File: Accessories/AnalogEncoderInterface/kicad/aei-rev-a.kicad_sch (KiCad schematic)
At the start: 55 parts, among them J1 Screw_Terminal_01x06, J2 1935161, J3 Screw_Terminal_01x06, U1 INA2143U, U2 INA2143U, U3 LT1764EQ-1.5-PBF, U4 RJHSE5380

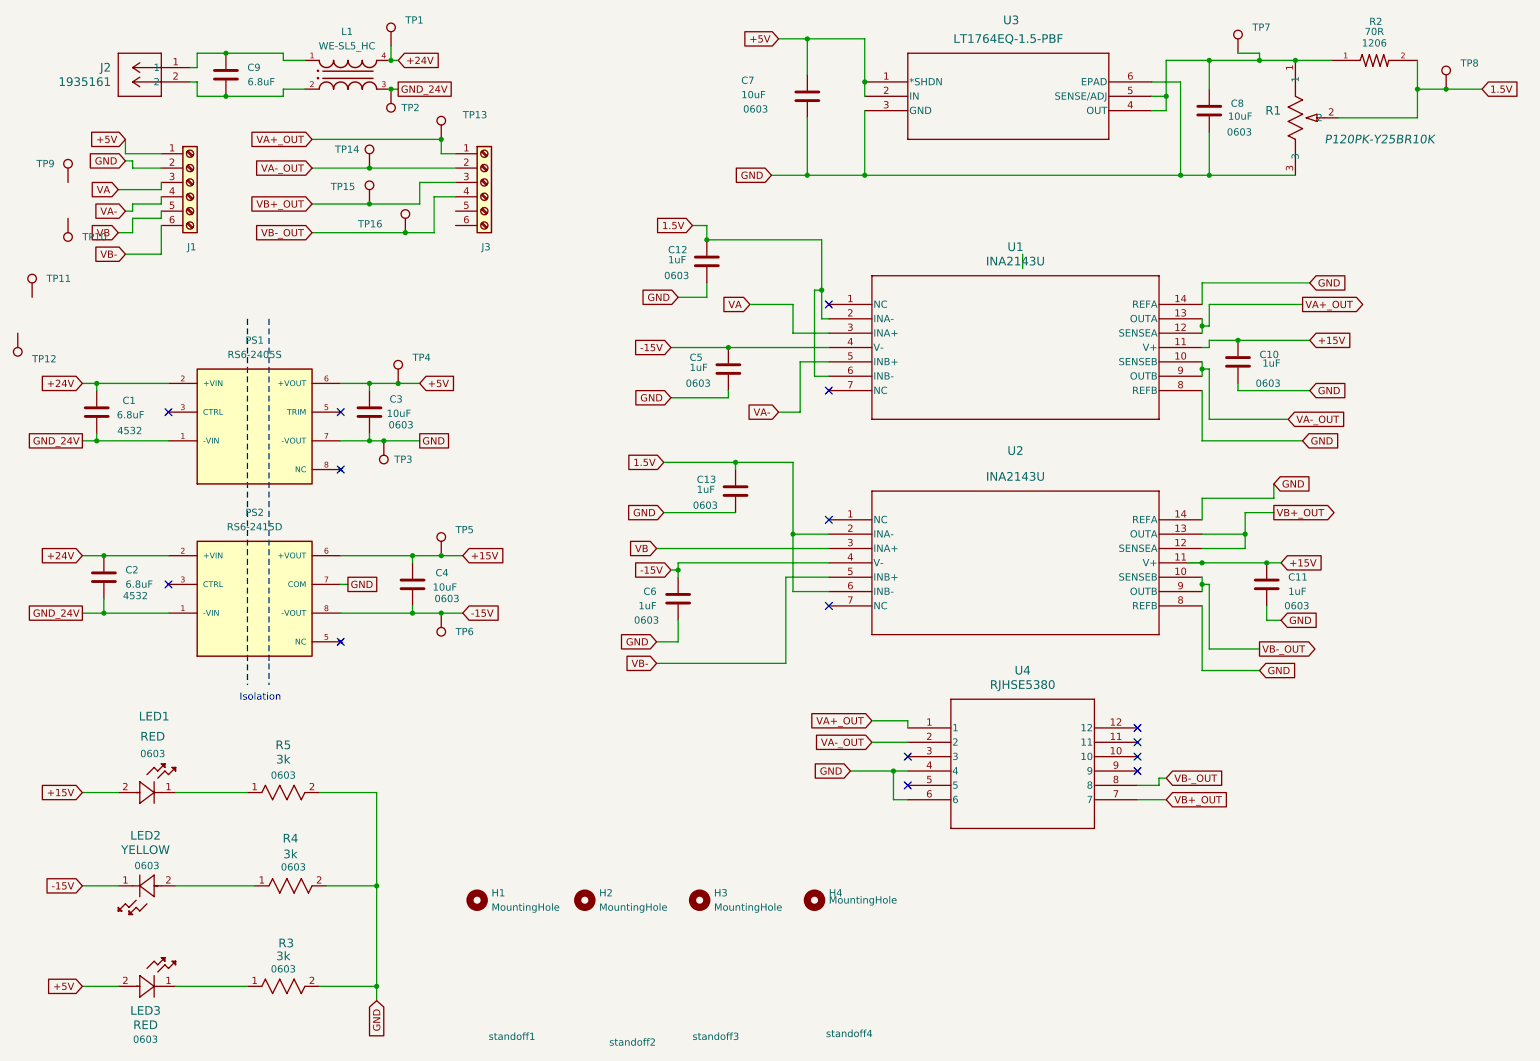
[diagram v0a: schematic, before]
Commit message: update the schematics
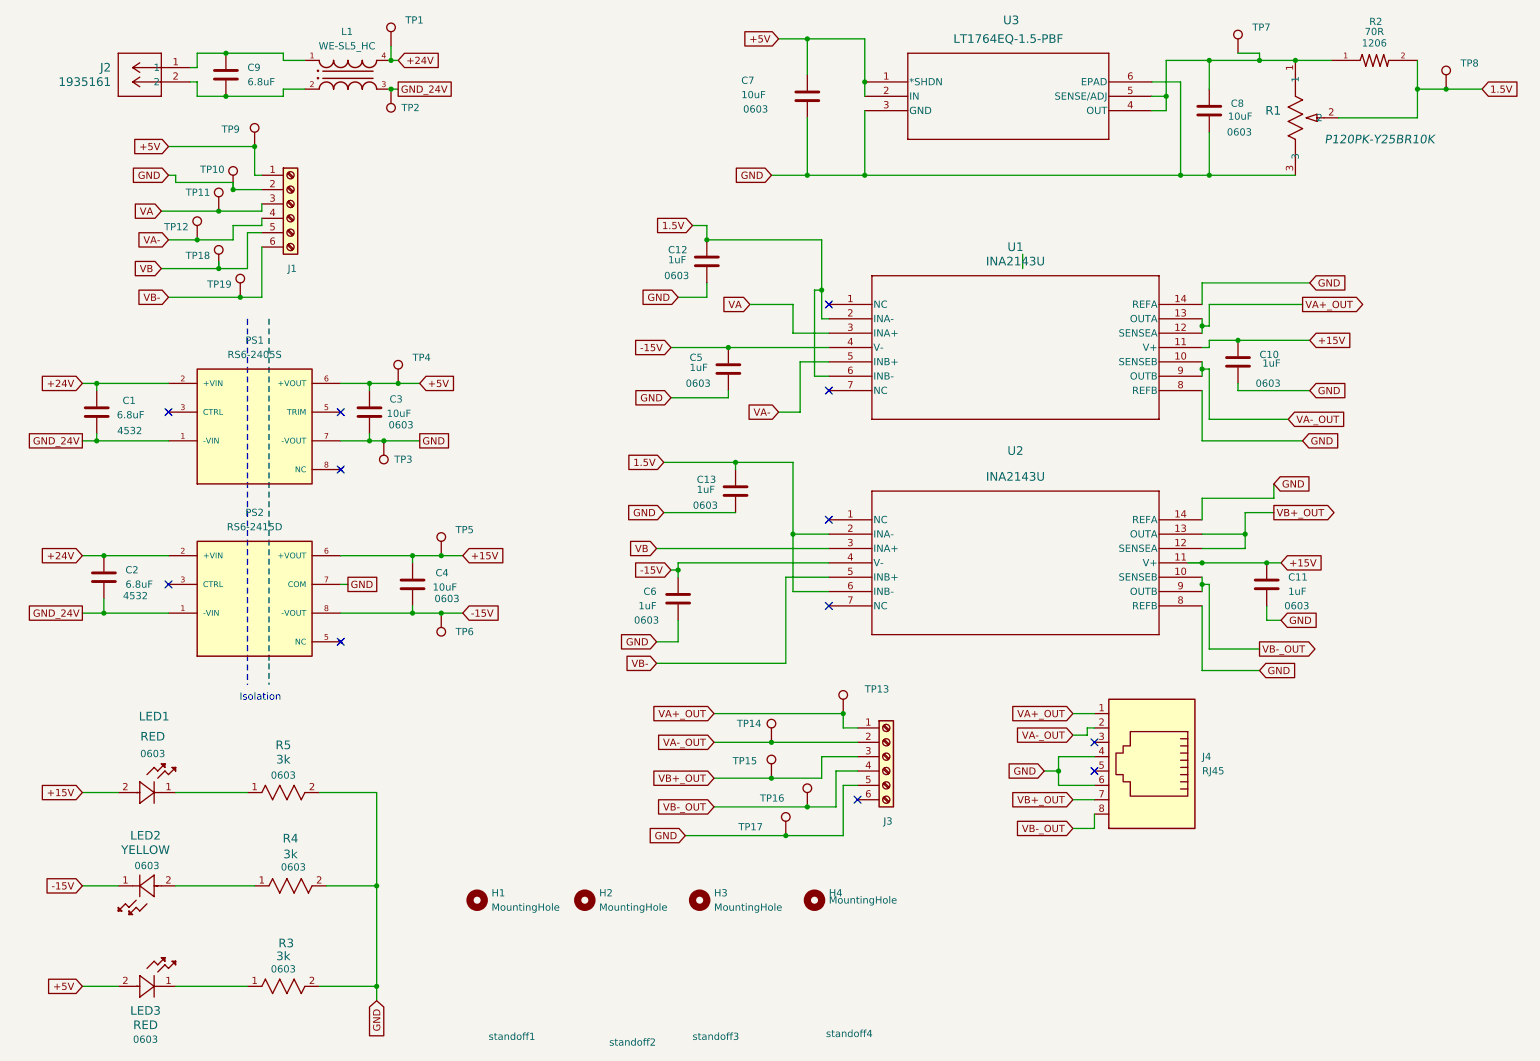
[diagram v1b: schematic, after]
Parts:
- removed U4: RJHSE5380, RJHSE5380:RJHSE5380_AMP, symbol RJHSE5380:RJHSE5380
- added J4: RJ45, symbol Connector:RJ45
- added TP17, TP18, TP19: TestPoint, symbol Connector:TestPoint
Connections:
- net +5V: now also TP9.1
- net GND: now also J3.5 (Pin_5), TP10.1, J4.4, J4.6, TP17.1
- net VA: now also TP11.1
- net VA+_OUT: now also J4.1
- net VA-: now also TP12.1
- net VA-_OUT: now also J4.2
- net VB: now also TP18.1
- net VB+_OUT: now also J4.7
- net VB-: now also TP19.1
- net VB-_OUT: now also J4.8
- no-connect marks 15 -> 12
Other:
- moved on the sheet: J1, J3, TP10, TP11, TP12, TP13, TP14, TP15, TP16, TP9
